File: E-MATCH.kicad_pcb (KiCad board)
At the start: 2 copper layers, 7 parts, among them IC1 NCV81071BZR2G, J2 691137710002, Q2 AOSP36326C, U1 TMCS1108A2UQDR

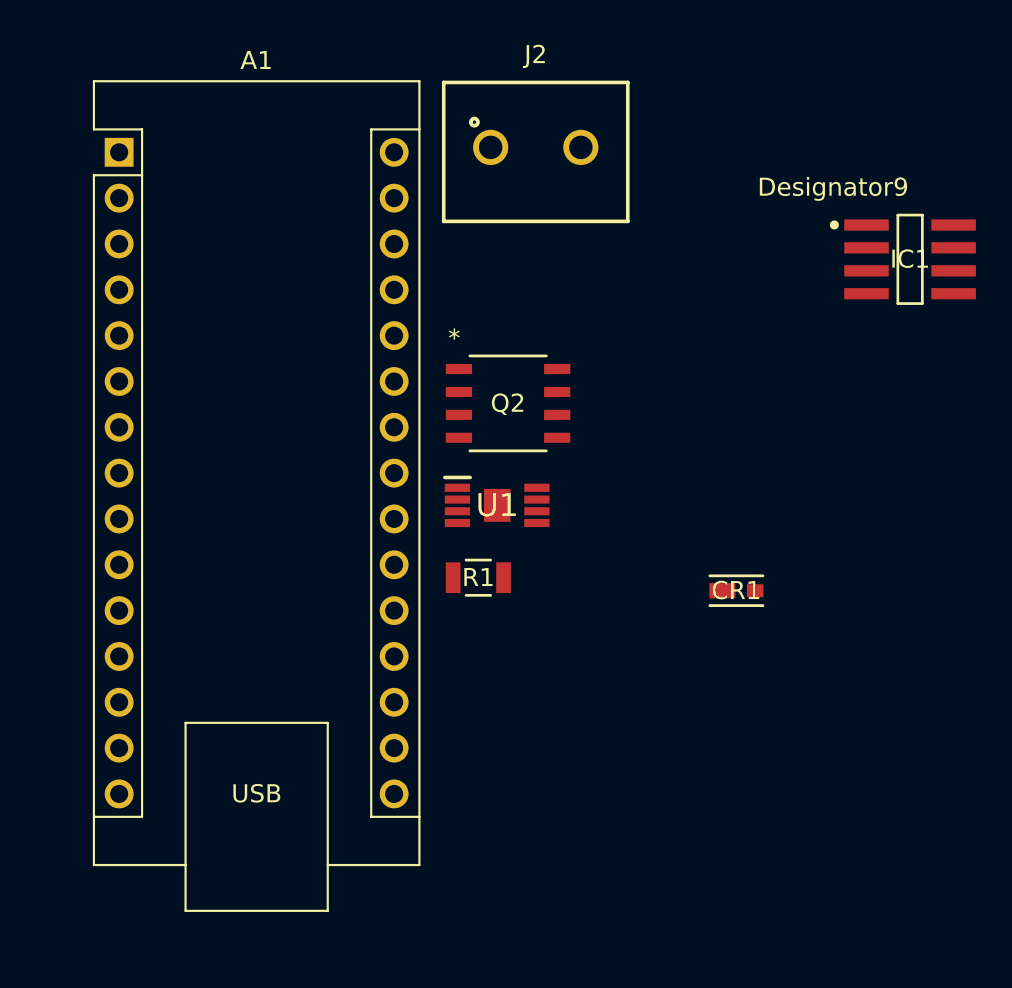
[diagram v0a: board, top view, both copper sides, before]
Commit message: linked 3-d models
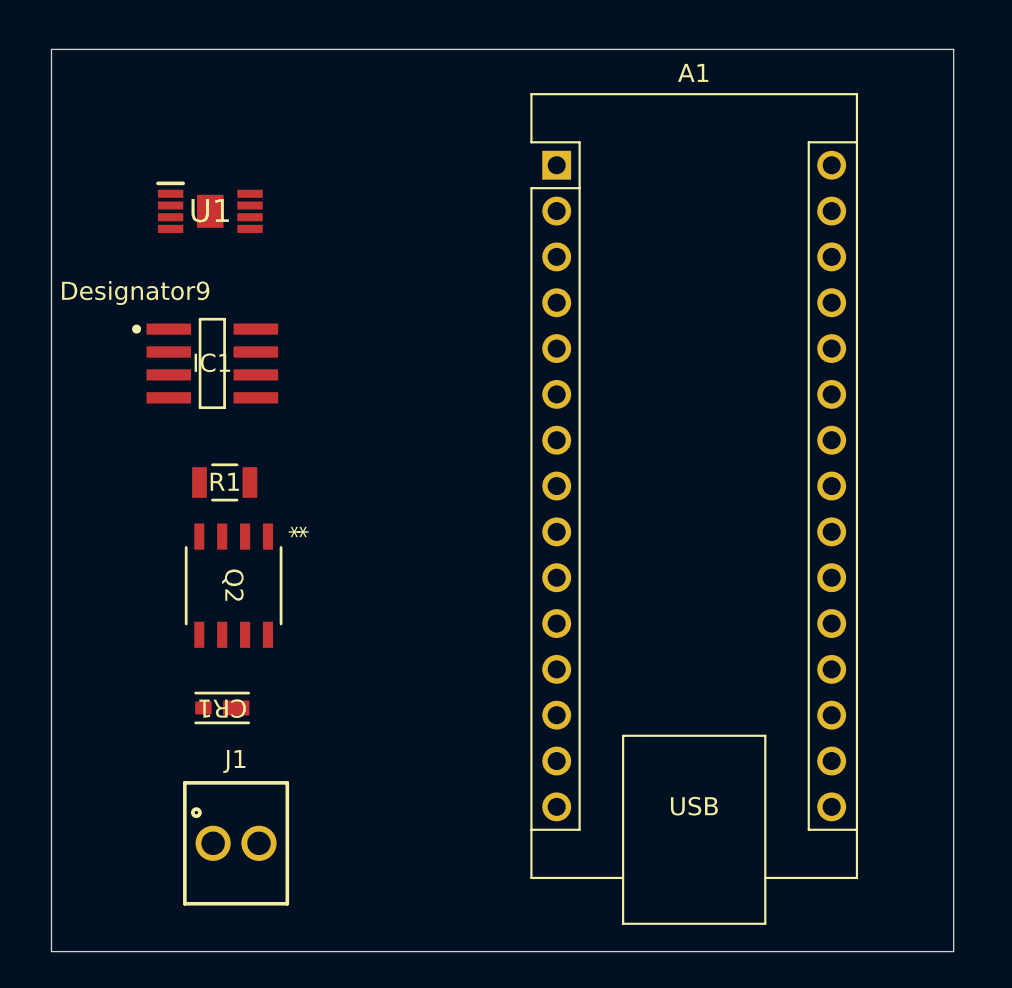
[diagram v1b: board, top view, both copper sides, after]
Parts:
- removed J2: 691137710002, Screw_Terminal_0102:691137710002
- added J1: 691210910002, Screw_Terminal:691210910002, F.Cu at (146.7, 114.5)
- moved IC1 39.1 mm to (145.4, 87.9)
- moved CR1 29.2 mm to (146.0, 107.0), turned to 180 degrees
- moved A1 24.3 mm to (164.5, 76.9)
- moved U1 22.8 mm to (145.3, 79.5)
- moved Q2 18.3 mm to (146.6, 100.2), turned to -90 degrees
- moved R1 15.0 mm to (146.1, 94.5)
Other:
- board outline added: 50 x 50 mm
